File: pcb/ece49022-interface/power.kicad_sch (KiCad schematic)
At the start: 13 parts, among them U5 TPS54202DDCT

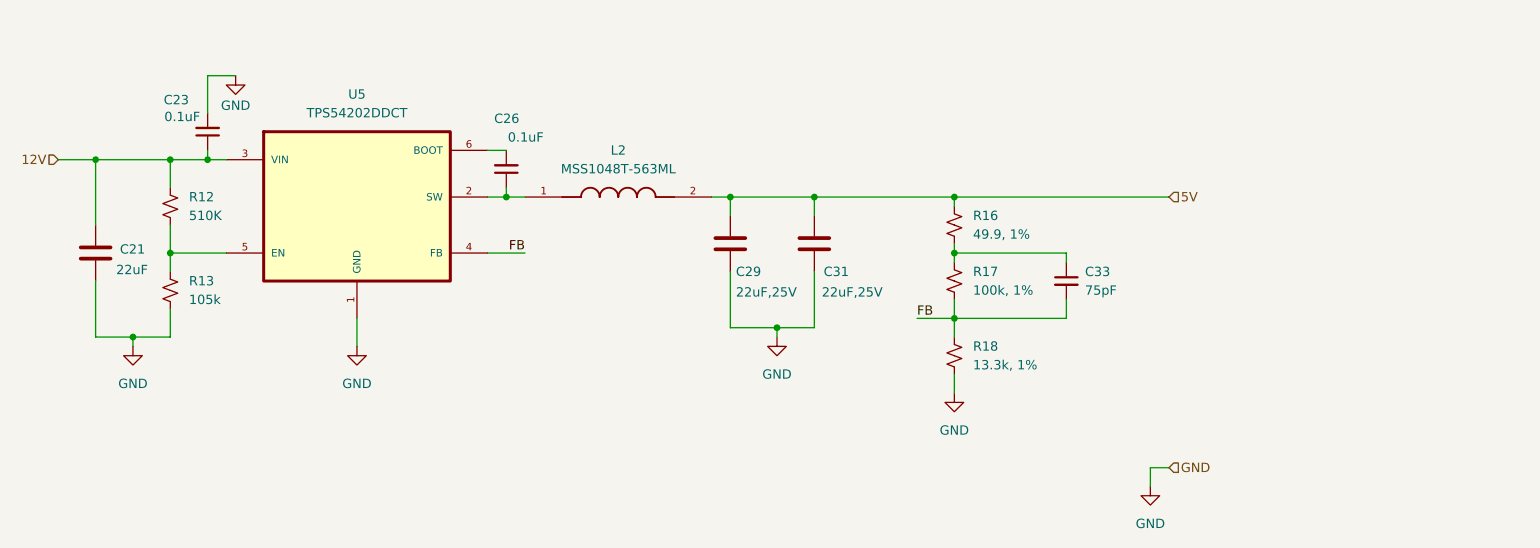
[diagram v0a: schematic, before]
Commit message: update
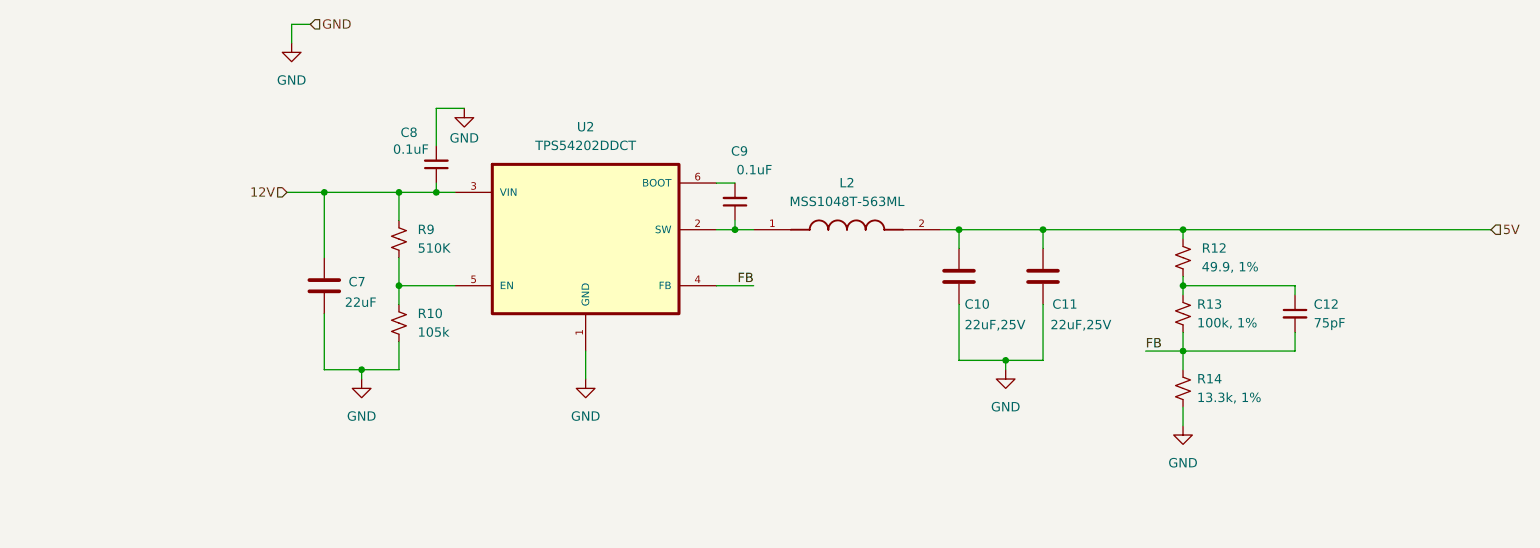
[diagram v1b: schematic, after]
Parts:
- removed C21: 22uF, Capacitor_SMD:C_0805_2012Metric_Pad1.18x1.45mm_HandSolder, symbol Device:C
- removed C23, C26: 0.1uF, Capacitor_SMD:C_0402_1005Metric, symbol Device:C_Small
- removed C29, C31: 22uF,25V, Capacitor_SMD:C_0805_2012Metric_Pad1.18x1.45mm_HandSolder, symbol Device:C
- removed C33: 75pF, Capacitor_SMD:C_0402_1005Metric, symbol Device:C_Small
- removed R16: 49.9, 1%, Capacitor_SMD:C_0402_1005Metric, symbol Device:R_Small_US
- removed R17: 100k, 1%, Capacitor_SMD:C_0402_1005Metric, symbol Device:R_Small_US
- removed R18: 13.3k, 1%, Capacitor_SMD:C_0402_1005Metric, symbol Device:R_Small_US
- removed U5: TPS54202DDCT, 49022_Footprints:TPS54202, symbol ECE49022_Symbols:TPS54202DDCT
- added C10, C11: 22uF,25V, Capacitor_SMD:C_0805_2012Metric_Pad1.18x1.45mm_HandSolder, symbol Device:C
- added C12: 75pF, Capacitor_SMD:C_0402_1005Metric, symbol Device:C_Small
- added C7: 22uF, Capacitor_SMD:C_1206_3216Metric, symbol Device:C
- added C8, C9: 0.1uF, Capacitor_SMD:C_0402_1005Metric, symbol Device:C_Small
- added R10: 105k, Capacitor_SMD:C_0402_1005Metric, symbol Device:R_Small_US
- added R14: 13.3k, 1%, Capacitor_SMD:C_0402_1005Metric, symbol Device:R_Small_US
- added R9: 510K, Capacitor_SMD:C_0402_1005Metric, symbol Device:R_Small_US
- added U2: TPS54202DDCT, 49022_Footprints:TPS54202, symbol ECE49022_Symbols:TPS54202DDCT
- R12: value 510K -> 49.9, 1%
- R13: value 105k -> 100k, 1%
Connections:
- net 12V: now also C7.1, C8.1, R9.1, U2.3 (VIN); no longer R12.1
- net 5V: now also R12.1, C10.1, C11.1
- net FB: now also R13.2, C12.2, R14.1, U2.4 (FB)
- net GND: now also C10.2, C11.2, C7.2, C8.2, R10.2, R14.2, U2.1 (GND); no longer R13.2
- net at R12.2, R13.1: now also C12.1
- net at L2.1: now also C9.1, U2.2 (SW)
- new net: C9.2, U2.6 (BOOT)
- new net: R10.1, R9.2, U2.5 (EN)
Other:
- moved on the sheet: L2
